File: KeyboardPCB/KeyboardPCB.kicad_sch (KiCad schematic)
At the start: 3 parts, among them P1 USB_C_Plug, P2 USB_C_Plug

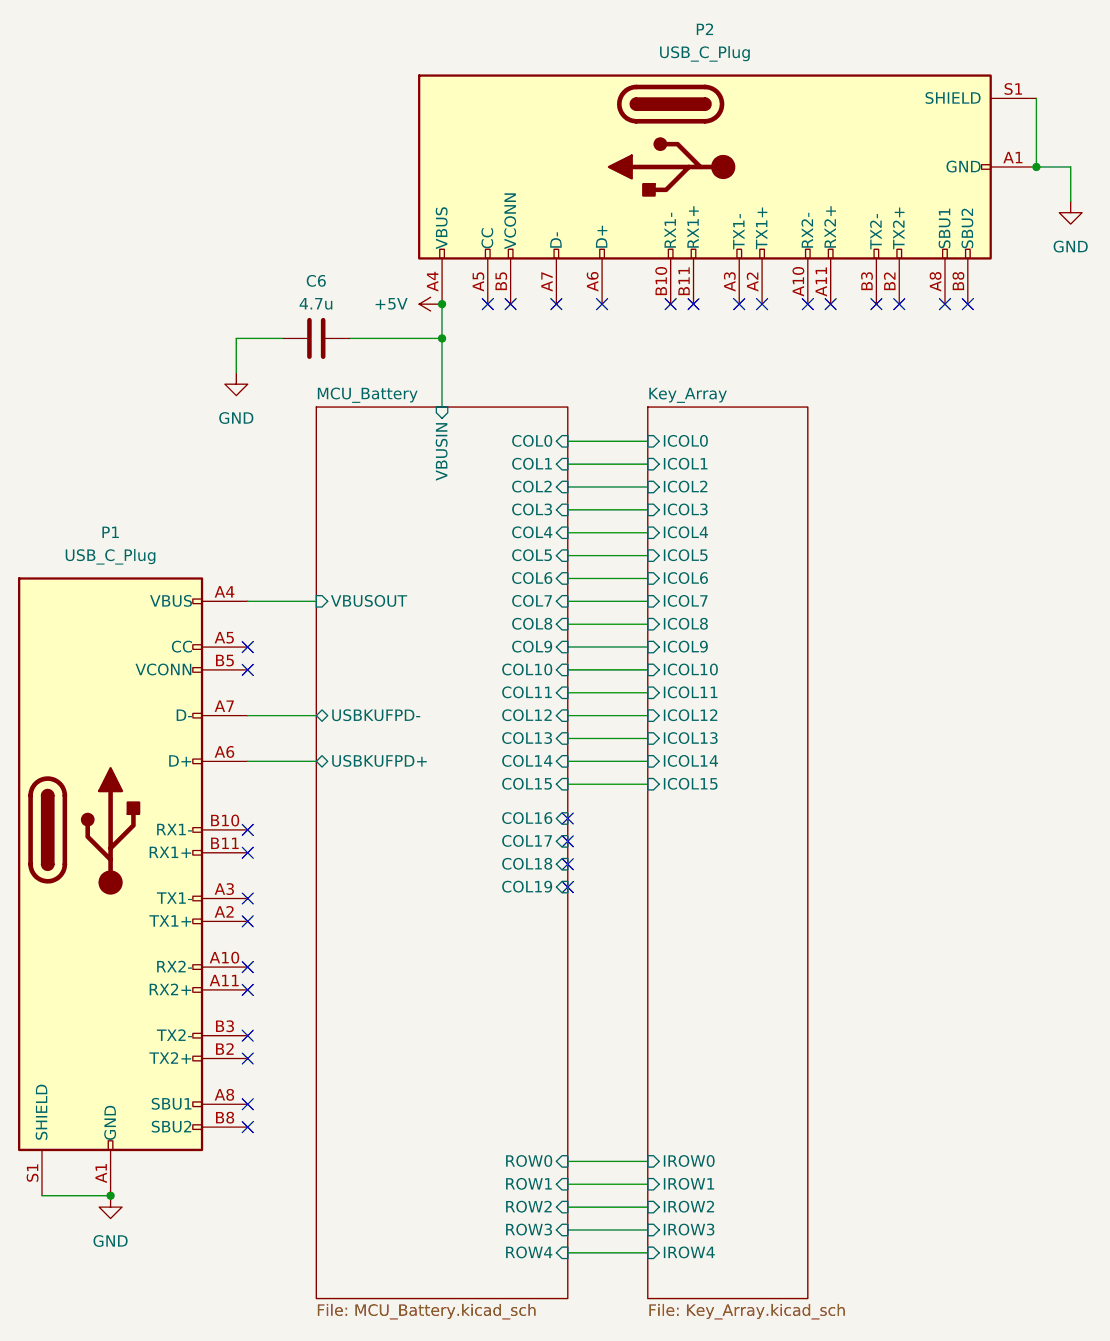
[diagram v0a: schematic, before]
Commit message: changed several components
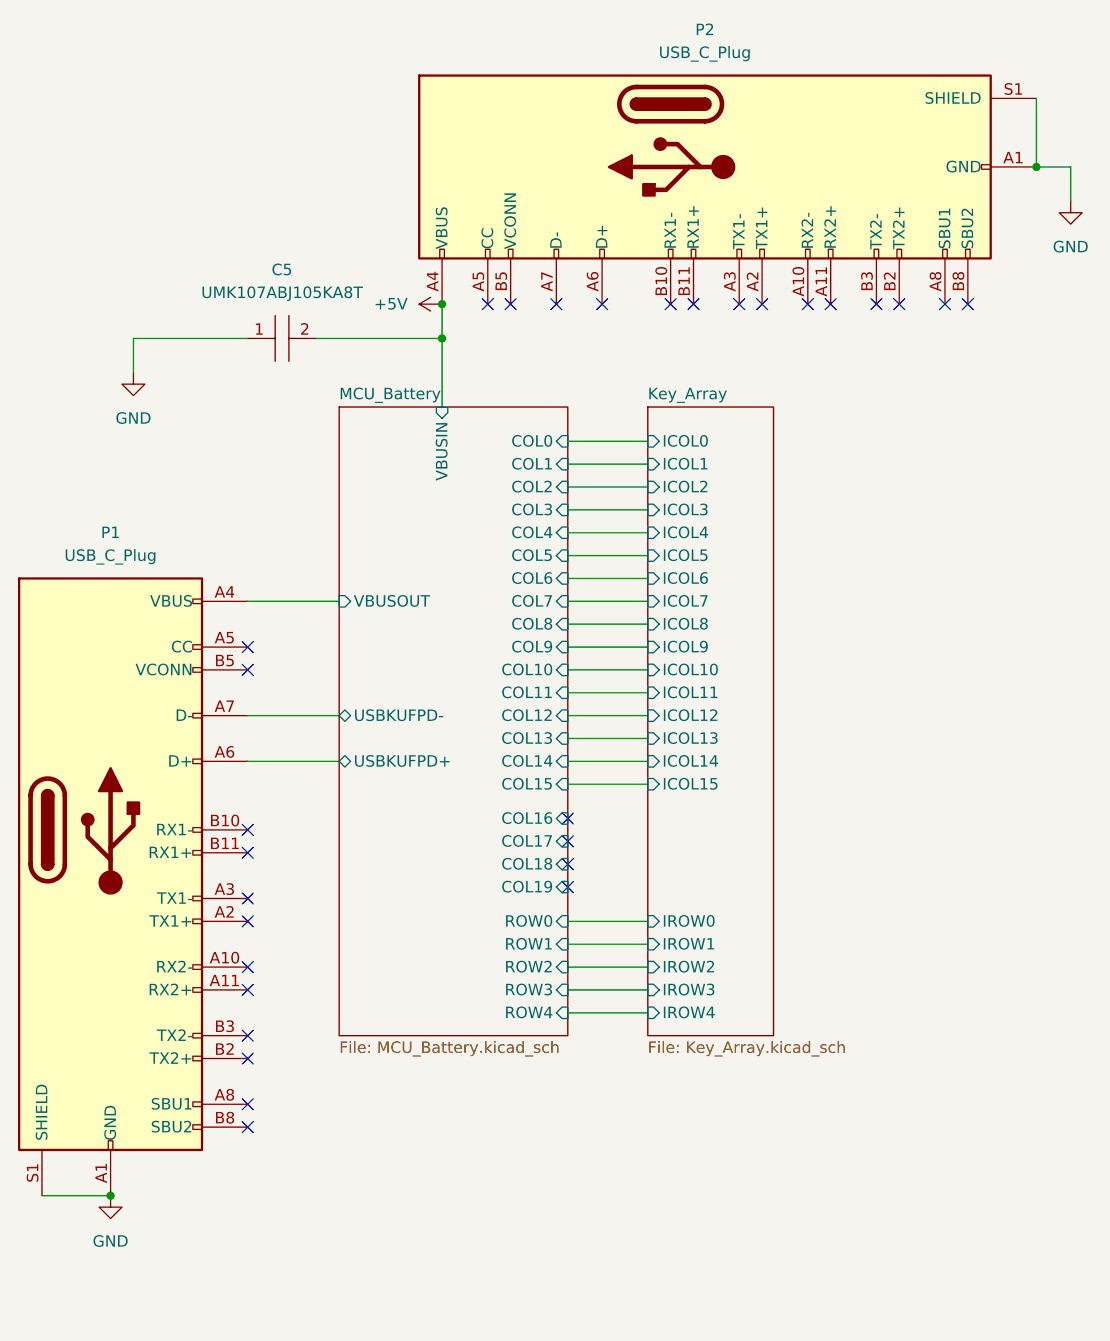
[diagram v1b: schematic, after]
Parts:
- removed C6: 4.7u, symbol Device:C
- added C5: UMK107ABJ105KA8T, keyboard_syms:CAPC1608X95N, symbol keyboard_syms:UMK107ABJ105KA8T
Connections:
- net +5V: now also C5.2
- net GND: now also C5.1
